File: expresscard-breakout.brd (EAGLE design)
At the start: 17.4 x 29.2 mm, 3 parts

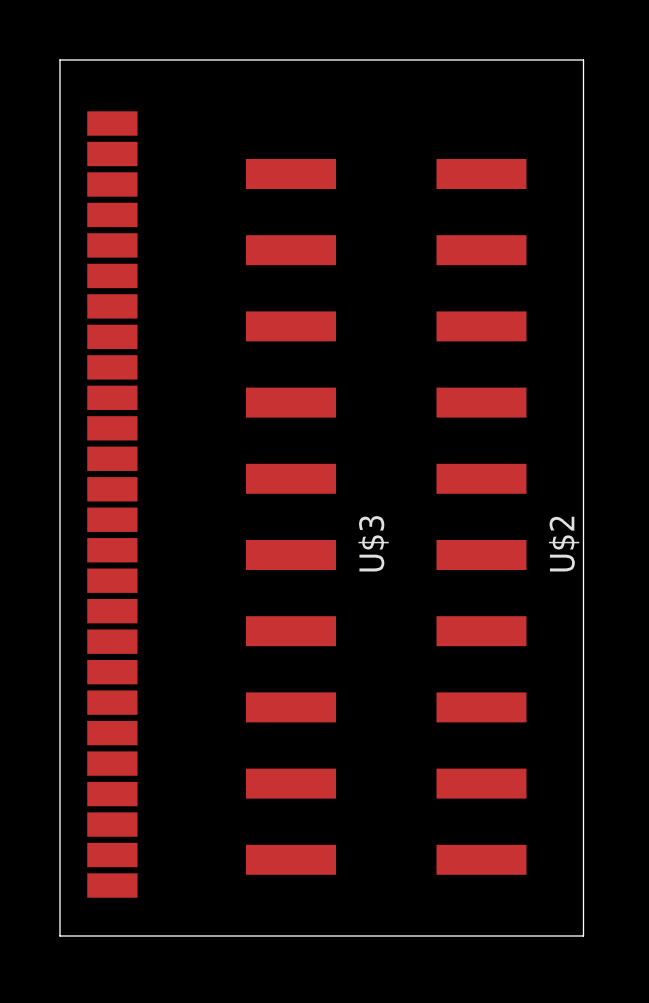
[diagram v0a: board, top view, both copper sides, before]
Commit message: I think it is done
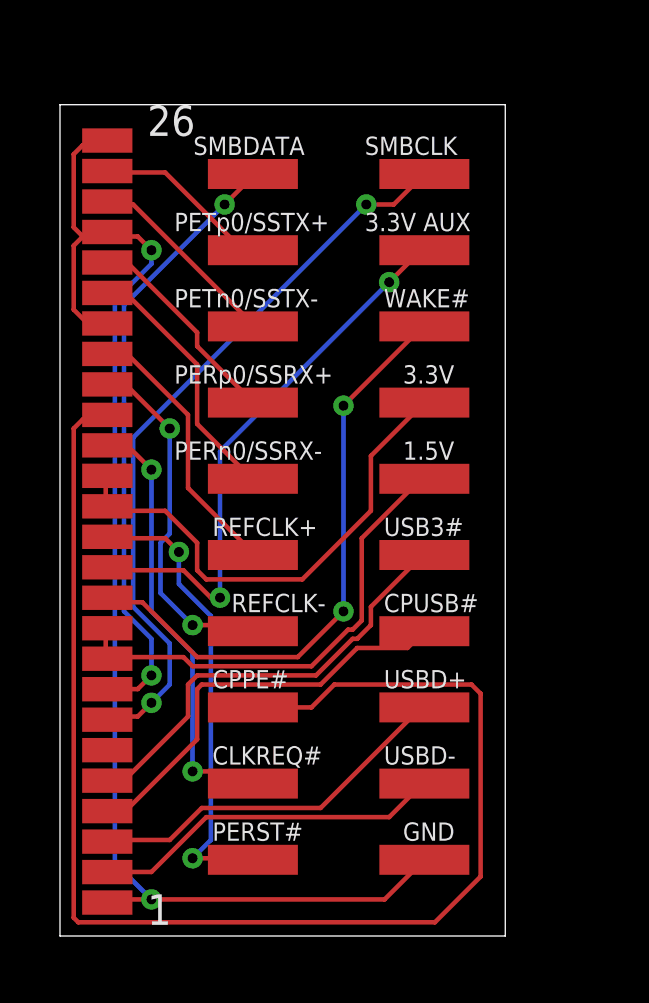
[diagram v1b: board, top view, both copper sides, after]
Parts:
- moved U$1 5.09 mm to (1.64, 14.0)
- moved U$2 1.91 mm to (17.1, 14.0)
- moved U$3 1.27 mm to (11.4, 14.0)
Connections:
- removed net 1.5V_A: U$1.P$9
- removed net 1.5V_B: U$1.P$10
- removed net 3.3V_A: U$1.P$14
- removed net 3.3V_AUX: U$1.P$12
- removed net 3.3V_B: U$1.P$15
- removed net GND_A: U$1.P$1
- removed net GND_B: U$1.P$20
- removed net GND_C: U$1.P$23
- removed net GND_D: U$1.P$26
- new net GND: U$1.P$1, U$1.P$20, U$1.P$23, U$1.P$26, U$2.1
- new net N$1: U$1.P$10, U$1.P$9, U$2.6
- new net N$10: U$1.P$7, U$2.10
- new net N$11: U$1.P$8, U$3.10
- new net N$12: U$1.P$13, U$3.1
- new net N$13: U$1.P$16, U$3.2
- new net N$14: U$1.P$17, U$3.3
- new net N$15: U$1.P$18, U$3.4
- new net N$16: U$1.P$19, U$3.5
- new net N$17: U$1.P$21, U$3.6
- new net N$18: U$1.P$22, U$3.7
- new net N$19: U$1.P$24, U$3.8
- new net N$20: U$1.P$25, U$3.9
- new net N$3: U$1.P$2, U$2.2
- new net N$4: U$1.P$3, U$2.3
- new net N$5: U$1.P$4, U$2.4
- new net N$6: U$1.P$5, U$2.5
- new net N$7: U$1.P$14, U$1.P$15, U$2.7
- new net N$8: U$1.P$11, U$2.8
- new net N$9: U$1.P$12, U$2.9
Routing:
- net N$14: track 0.00 -> 46.0 mm
- net GND: track 0.00 -> 45.4 mm, vias 0 -> 2
- net N$10: track 0.00 -> 24.6 mm, vias 0 -> 2
- net N$11: track 0.00 -> 20.5 mm, vias 0 -> 2
- net N$8: track 0.00 -> 20.0 mm, vias 0 -> 2
- net N$9: track 0.00 -> 18.6 mm, vias 0 -> 2
- net N$7: track 0.00 -> 16.7 mm
- net N$1: track 0.00 -> 16.0 mm
- net N$12: track 0.00 -> 15.5 mm, vias 0 -> 2
- net N$6: track 0.00 -> 14.7 mm
- net N$13: track 0.00 -> 14.6 mm, vias 0 -> 2
- net N$5: track 0.00 -> 14.0 mm
- net N$4: track 0.00 -> 12.4 mm
- net N$15: track 0.00 -> 11.9 mm, vias 0 -> 2
- net N$3: track 0.00 -> 11.8 mm
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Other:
- board size 17.4 x 29.2 mm -> 14.8 x 27.7 mm
- board text added: "1.5V"
- board text added: "20151106"
- board text added: "3.3V"
- board text added: "3.3V AUX"
- board text added: "CLKREQ#"
- board text added: "CPPE#"
- board text added: "CPUSB#"
- board text added: "ExpressCard34 Breakout"
- board text added: "GND"
- board text added: "HokieGeek"
- board text added: "PERST#"
- board text added: "PERn0/SSRX-"
- board text added: "PERp0/SSRX+"
- board text added: "PETn0/SSTX-"
- board text added: "PETp0/SSTX+"
- board text added: "REFCLK+"
- board text added: "REFCLK-"
- board text added: "SMBCLK"
- board text added: "SMBDATA"
- board text added: "USB3#"
- board text added: "USBD+"
- board text added: "USBD-"
- board text added: "WAKE#"
